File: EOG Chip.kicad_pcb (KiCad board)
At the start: 2 copper layers, 17 parts, among them U1 INA128, U2 INA128, U3 TL074, U4 STM32WB55CCUx

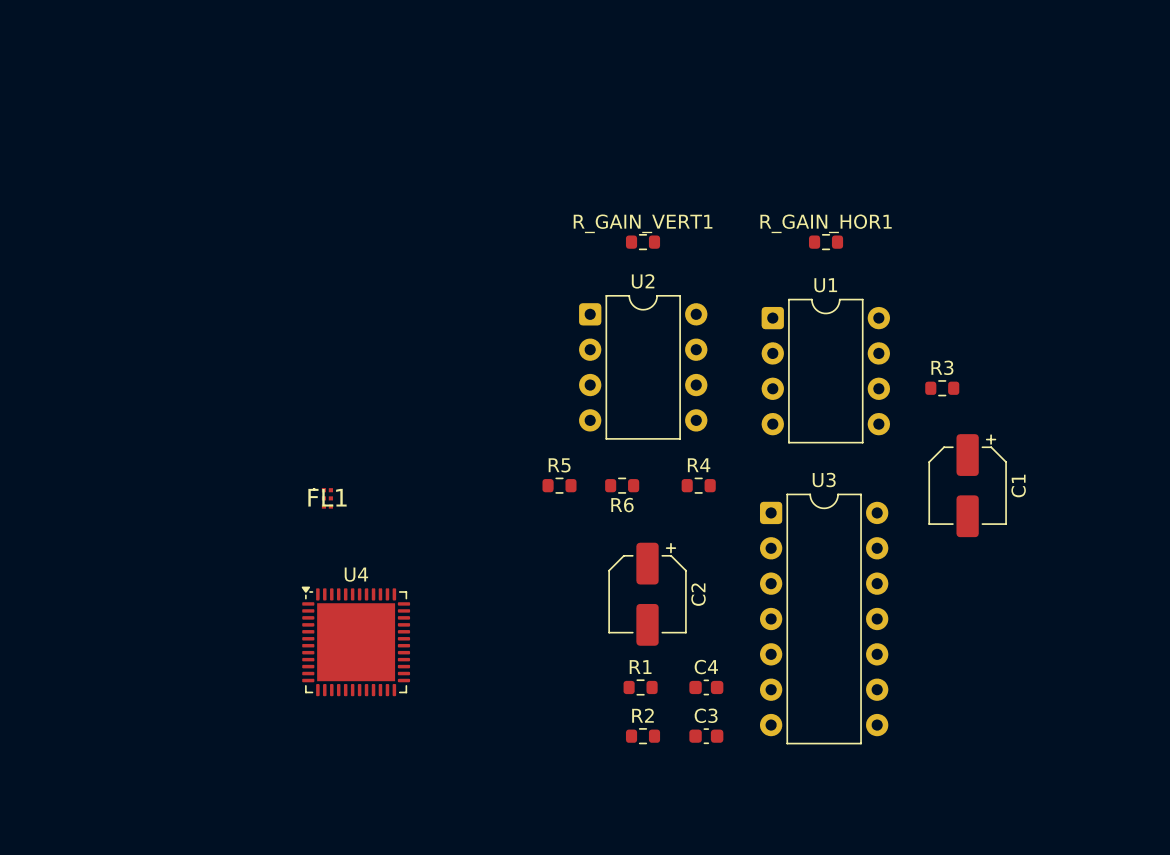
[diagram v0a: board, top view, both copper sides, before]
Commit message: updated files
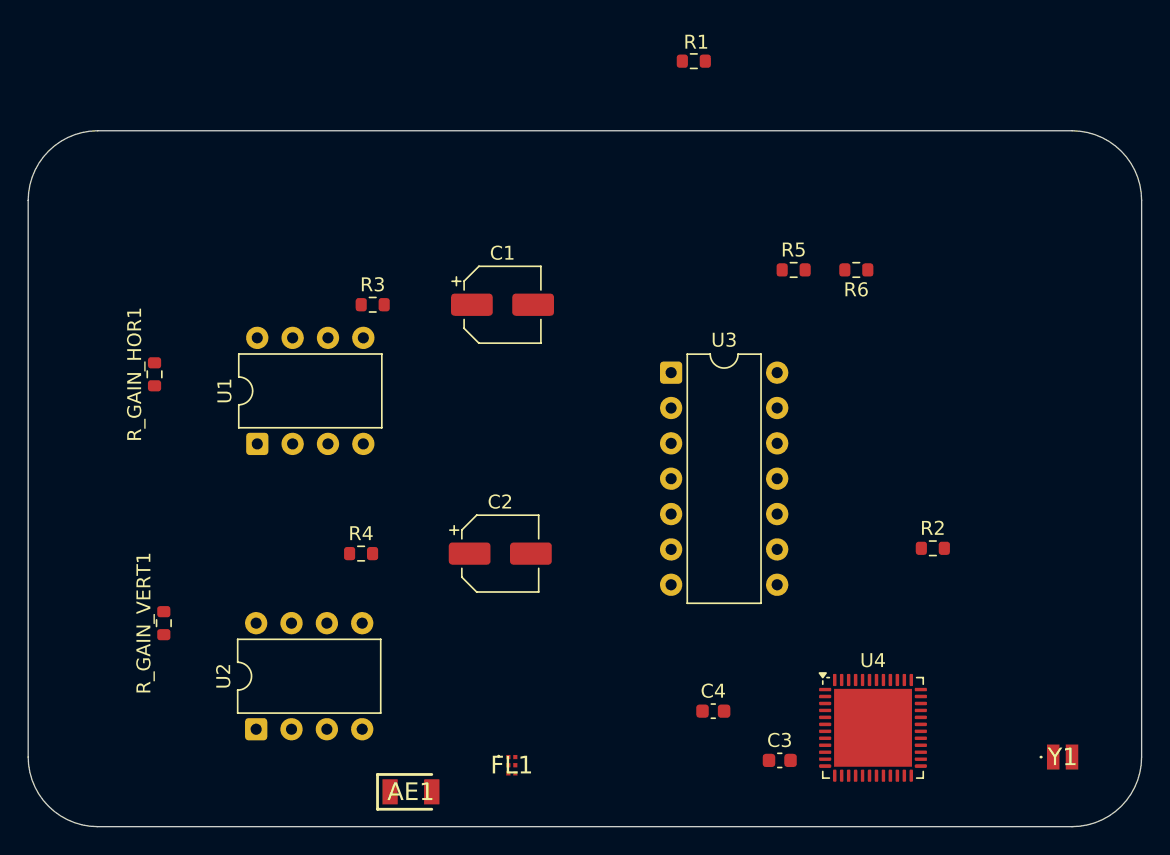
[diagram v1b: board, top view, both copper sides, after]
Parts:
- added AE1: Antenna, antenna_ghz:ANTC3216X60N, F.Cu at (132.5, 107.5)
- added Y1: Crystal, new_crystal:ABM11A32000MHZD2YT3, F.Cu at (179.3, 105.0)
- FL1: footprint AntennaFilter_MLPF:BUMPLESS_CSP_2025 -> a_rf_module:BUMPLESS_CSP_2025
- moved R_GAIN_HOR1 49.2 mm to (114.1, 77.5), turned to 90 degrees
- moved R1 45.2 mm to (152.8, 55.0)
- moved R_GAIN_VERT1 44.0 mm to (114.7, 95.4), turned to 90 degrees
- moved R3 41.4 mm to (129.8, 72.5)
- moved U2 38.3 mm to (121.4, 103.0), turned to 90 degrees
- moved U1 38.1 mm to (121.5, 82.5), turned to 90 degrees
- moved U4 37.6 mm to (165.7, 102.9)
- moved C1 35.9 mm to (139.1, 72.5), turned to 0 degrees
- moved R2 24.8 mm to (170.0, 90.0)
- moved R4 24.7 mm to (128.9, 90.4)
- moved FL1 23.3 mm to (139.8, 105.6)
- moved R5 22.9 mm to (160.0, 70.0)
- moved R6 22.9 mm to (164.5, 70.0)
- moved U3 12.4 mm to (151.2, 77.4)
- moved C2 11.0 mm to (138.9, 90.4), turned to 0 degrees
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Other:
- board outline added: 80 x 50 mm

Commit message: updating schematics
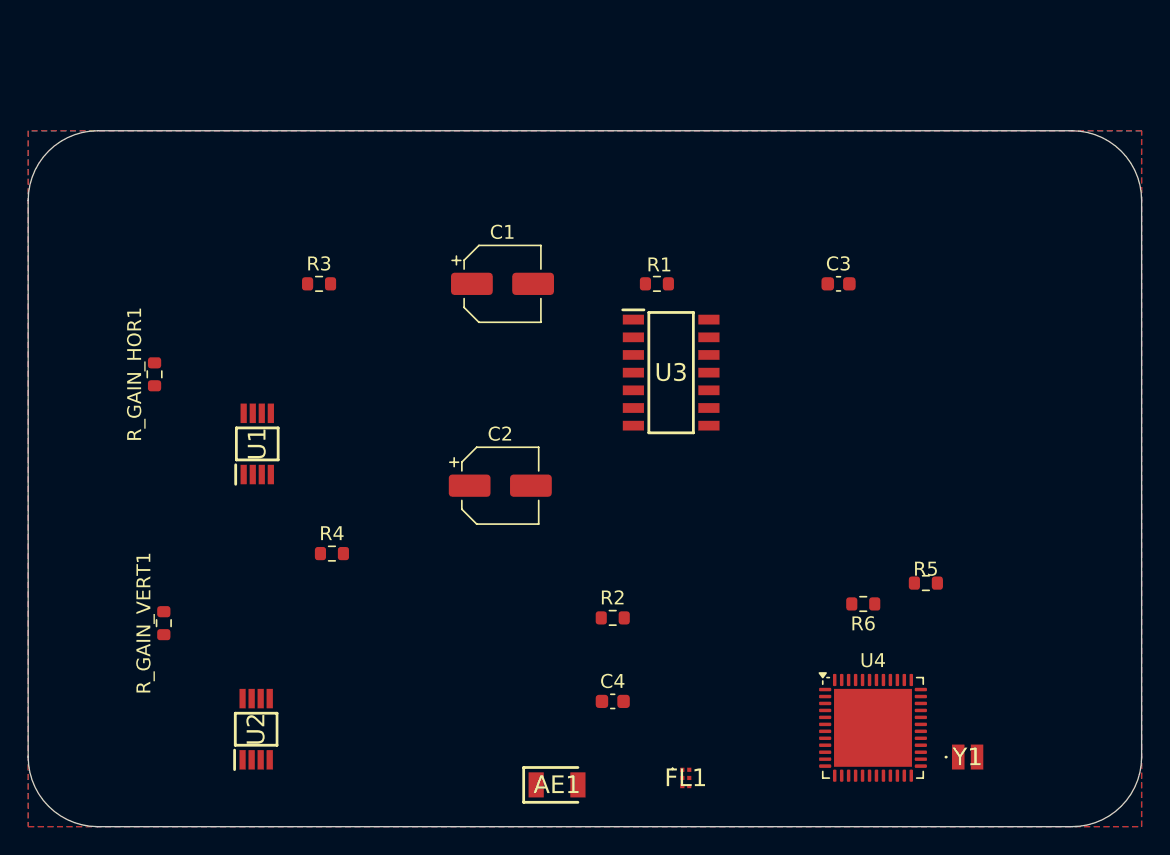
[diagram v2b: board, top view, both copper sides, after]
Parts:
- U1, U2: footprint Package_DIP:DIP-8_W7.62mm -> amp_new:SOP65P490X110-8N
- U3: footprint Package_DIP:DIP-14_W7.62mm -> amp_new_big:SOIC127P600X175-14N
- moved C3 34.5 mm to (163.2, 71.0)
- moved R5 24.4 mm to (169.5, 92.5)
- moved R6 24.0 mm to (165.0, 94.0)
- moved R2 23.5 mm to (147.0, 95.0)
- moved R1 16.2 mm to (150.2, 71.0)
- moved FL1 12.5 mm to (152.2, 106.5)
- moved AE1 10.5 mm to (143.0, 107.0)
- moved C4 7.26 mm to (147.0, 101.0)
- moved Y1 6.82 mm to (172.5, 105.0)
- moved C2 4.88 mm to (138.9, 85.5)
- moved R3 4.14 mm to (125.9, 71.0)
- moved R4 2.09 mm to (126.8, 90.4)
- moved C1 1.50 mm to (139.1, 71.0)
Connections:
- U3 pad 13: Net-(U2-Ref) -> Net-(U1-Ref)
- U3 pad 14: Net-(U2-Ref) -> Net-(U1-Ref)
- U3 pad 8: Net-(U1-Ref) -> Net-(U2-Ref)
- U3 pad 9: Net-(U1-Ref) -> Net-(U2-Ref)
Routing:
- added copper zone on B.Cu, net GND
- added copper zone on F.Cu, net GND
